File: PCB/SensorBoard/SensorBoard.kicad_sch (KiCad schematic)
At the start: 0 parts

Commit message: More main
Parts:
- added J1: Conn_02x04_Odd_Even, Connector_PinHeader_2.54mm:PinHeader_2x04_P2.54mm_Vertical, symbol Connector_Generic:Conn_02x04_Odd_Even
- added R1, R3, R5, R7, R9: 90, Resistor_SMD:R_0805_2012Metric, symbol Device:R
- added R10, R2, R4, R6, R8: 3.9k, Resistor_SMD:R_0805_2012Metric, symbol Device:R
- added U1, U2, U3, U4, U5: TCRT5000, kicad_mod:OPTO_TCRT5000, symbol TCRT5000:TCRT5000
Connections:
- new net: R7.1, U4.CATH
- new net: R1.1, U1.CATH
- new net: R9.1, U5.CATH
- new net: R5.1, U3.CATH
- new net: R3.1, U2.CATH
- new net +3.3V: J1.2 (Pin_2), U1.A, U1.COLL, U2.A, U2.COLL, U3.A, U3.COLL, U4.A, U4.COLL, U5.A, U5.COLL
- new net Analog Pin1: J1.1 (Pin_1), R2.1, U1.E
- new net Analog Pin2: J1.3 (Pin_3), R4.1, U2.E
- new net Analog Pin3: J1.5 (Pin_5), R6.1, U3.E
- new net Analog Pin4: J1.4 (Pin_4), R8.1, U4.E
- new net Analog Pin5: J1.6 (Pin_6), R10.1, U5.E
- new net GND: J1.7 (Pin_7), R1.2, R10.2, R2.2, R3.2, R4.2, R5.2, R6.2, R7.2, R8.2, R9.2

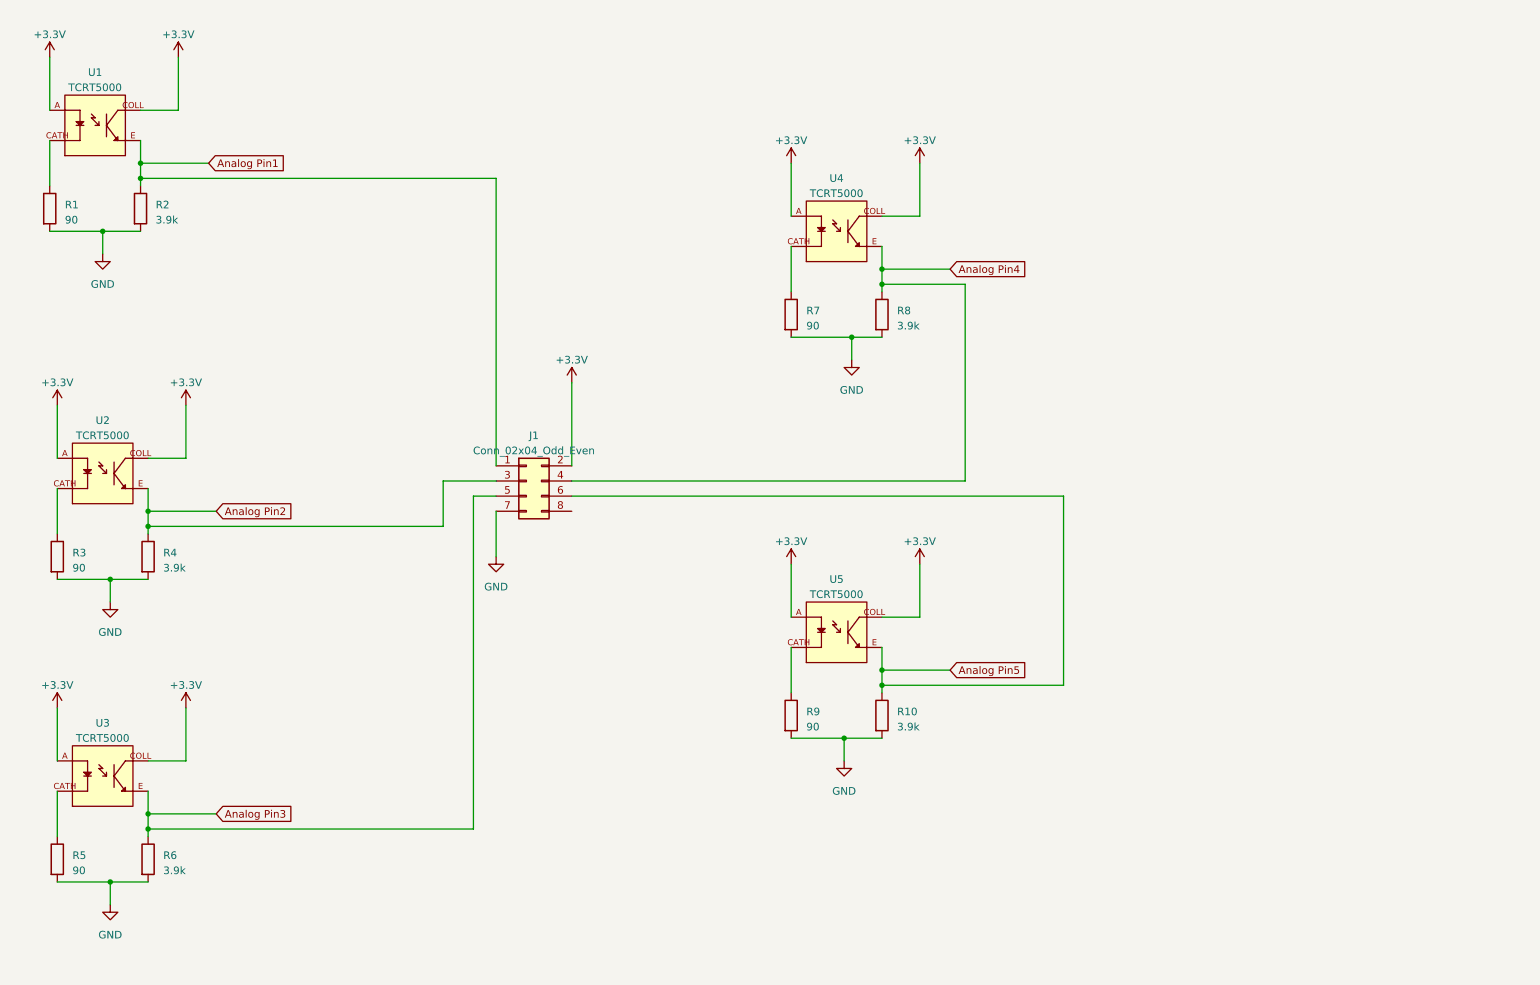
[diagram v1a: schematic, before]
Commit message: Cleaned up repo
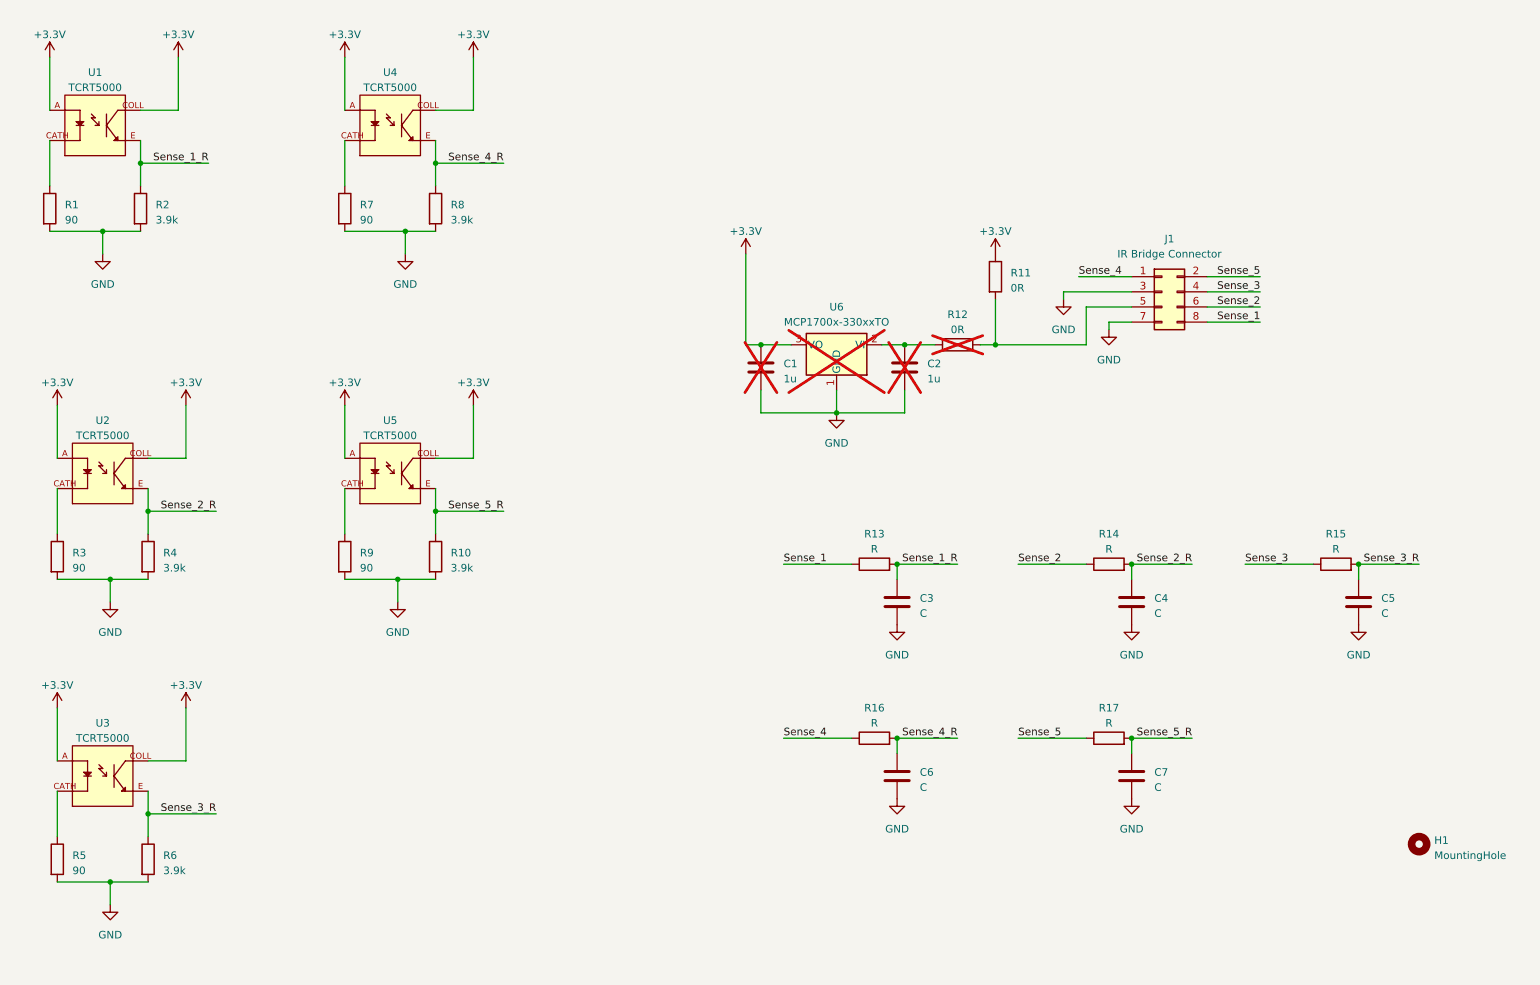
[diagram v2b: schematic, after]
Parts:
- added C1, C2: 1u, Capacitor_SMD:C_0603_1608Metric_Pad1.08x0.95mm_HandSolder, symbol Device:C
- added C3, C4, C5, C6, C7: C, Capacitor_SMD:C_1206_3216Metric, symbol Device:C
- added H1: MountingHole, MountingHole:MountingHole_2.2mm_M2, symbol Mechanical:MountingHole
- added R11, R12: 0R, Resistor_SMD:R_0805_2012Metric, symbol Device:R
- added R13, R14, R15, R16, R17: R, Resistor_SMD:R_0805_2012Metric, symbol Device:R
- added U6: MCP1700x-330xxTO, Package_TO_SOT_THT:TO-92_Inline, symbol Regulator_Linear:MCP1700x-330xxTO
- J1: value Conn_02x04_Odd_Even -> IR Bridge Connector
- U1, U2, U3, U4, U5: footprint kicad_mod:OPTO_TCRT5000 -> OptoDevice:OPTO_TCRT5000
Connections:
- net +3.3V: now also C1.1, R11.1, U6.3 (VO); no longer J1.2 (Pin_2)
- net GND: now also J1.3 (Pin_3), C1.2, C2.2, C3.2, C4.2, C5.2, C6.2, C7.2, U6.1 (GND)
- net Sense_1: now reaches J1.8 (Pin_8)
- net Sense_1: now also R13.1
- net Analog Pin1 renamed Sense_1_R
- net Sense_1_R: now also C3.1, R13.2; no longer J1.1 (Pin_1)
- net Analog Pin2 renamed Sense_2_R
- net Sense_2_R: now also C4.1, R14.2; no longer J1.3 (Pin_3)
- net Analog Pin3 renamed Sense_3_R
- net Sense_3_R: now also C5.1, R15.2; no longer J1.5 (Pin_5)
- net Analog Pin4 renamed Sense_4_R
- net Sense_4_R: now also C6.1, R16.2; no longer J1.4 (Pin_4)
- net Analog Pin5 renamed Sense_5_R
- net Sense_5_R: now also C7.1, R17.2; no longer J1.6 (Pin_6)
- new net: J1.5 (Pin_5), R11.2, R12.2
- new net: C2.1, R12.1, U6.2 (VI)
- new net Sense_2: J1.6 (Pin_6), R14.1
- new net Sense_3: J1.4 (Pin_4), R15.1
- new net Sense_4: J1.1 (Pin_1), R16.1
- new net Sense_5: J1.2 (Pin_2), R17.1
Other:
- moved on the sheet: J1, R10, R7, R8, R9, U4, U5

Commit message: Cleaned up sensor board
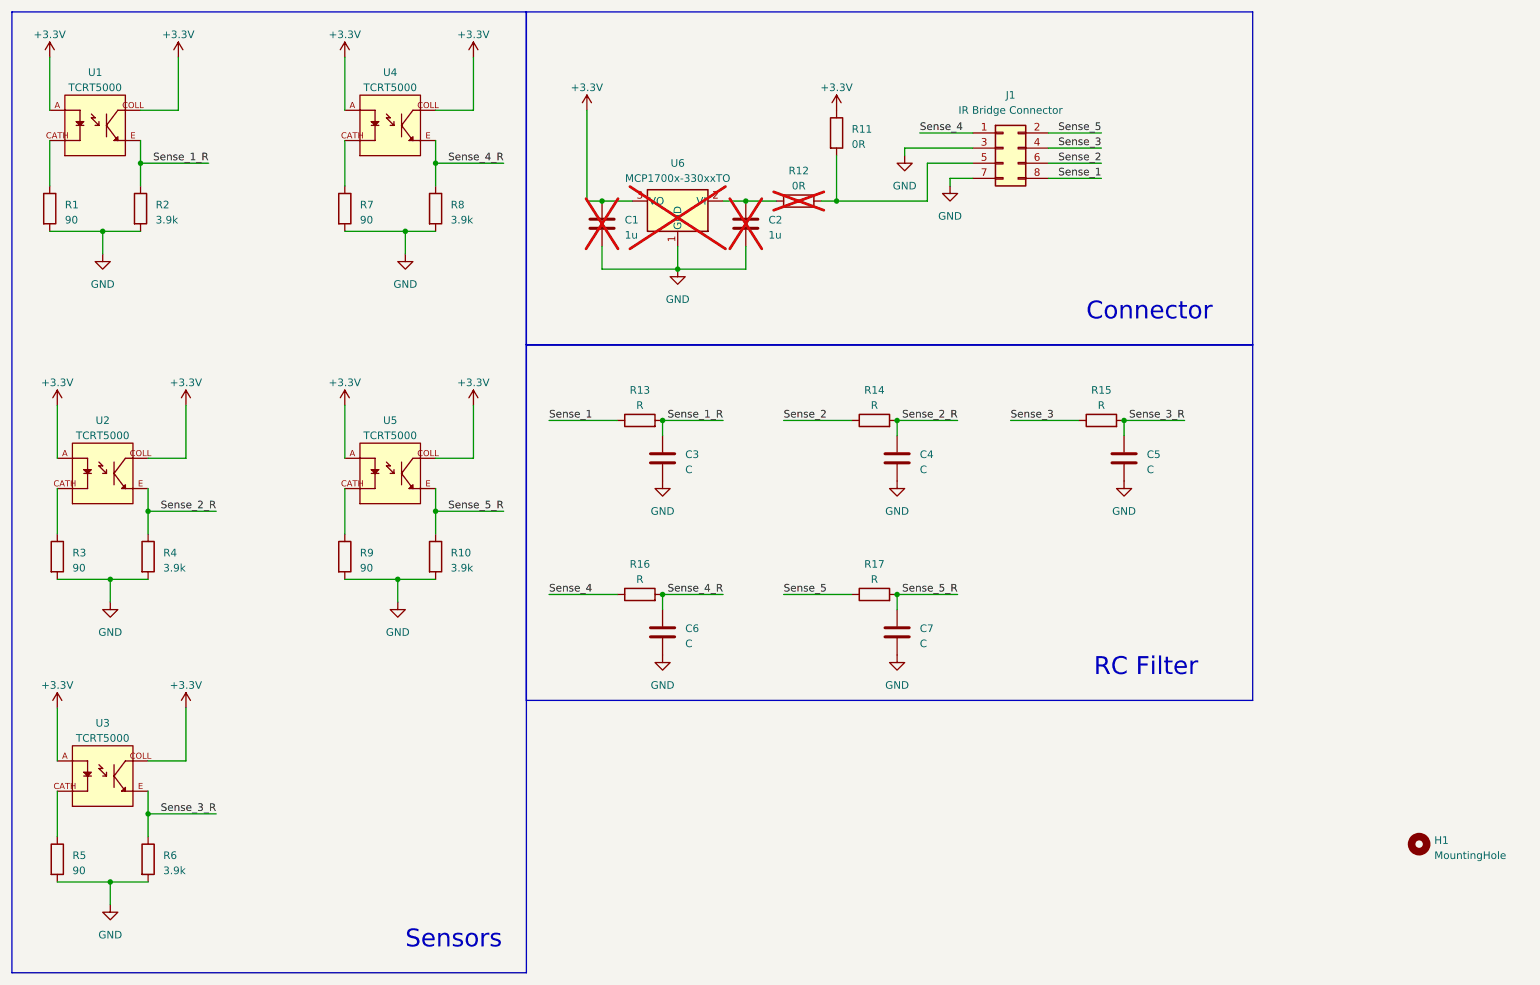
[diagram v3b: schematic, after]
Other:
- note added: "Connector"
- note added: "RC Filter"
- note added: "Sensors"
- moved on the sheet: C1, C2, C3, C4, C5, C6, C7, J1, R11, R12, R13, R14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
